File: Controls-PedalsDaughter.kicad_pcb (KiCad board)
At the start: 2 copper layers, 40 x 50 mm, 37 parts, among them J2 Accel Pos. Sensor, J3 PeripheralCANConnector, J4 Conn_01x02, J5 PeripheralCANConnector, U1 RI3-1205S, U2 PeripheralSOM, U3 TLV9301xDCK, U4 AMC1300BDWV, U5 TLV70130DBVR

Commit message: again
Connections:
- D1 pad 1: +3.3V -> +3V3
- D3 pad 1: +3.3V -> +3V3
- U2 pad 2: +3.3V -> +3V3
- U2 pad 9: +3.3V -> +3V3
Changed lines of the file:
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@@
 	(net 7 "+3V3PWR")
 	(net 8 "+3V3")
-	(net 9 "+3.3V")
-	(net 10 "Net-(D6-A)")
-	(net 11 "unconnected-(J2-Pin_2-Pad2)")
-	(net 12 "Net-(J2-Pin_5)")
-	(net 13 "/CAN_L")
-	(net 14 "/CAN_H")
-	(net 15 "/INP")
-	(net 16 "Net-(U3-+)")
-	(net 17 "unconnected-(U2-SPI1_NSS-Pad19)")
-	(net 18 "unconnected-(U2-I2C2_SCL-Pad8)")
-	(net 19 "unconnected-(U2-SPI1_MISO-Pad15)")
-	(net 20 "unconnected-(U2-VDDA(3.3V)-Pad10)")
-	(net 21 "unconnected-(U2-SPI2_NSS-Pad7)")
-	(net 22 "unconnected-(U2-GNDA-Pad12)")
-	(net 23 "unconnected-(U2-SPI1_SCK-Pad13)")
-	(net 24 "unconnected-(U2-SPI2_MOSI-Pad1)")
-	(net 25 "unconnected-(U2-SPI2_MISO-Pad3)")
-	(net 26 "unconnected-(U2-I2C1_SDA-Pad16)")
-	(net 27 "unconnected-(U2-I2C2_SDA-Pad6)")
-	(net 28 "unconnected-(U2-SPI2_SCK-Pad5)")
-	(net 29 "unconnected-(U2-SPI1_MOSI-Pad17)")
-	(net 30 "unconnected-(U2-I2C1_SCL-Pad14)")
-	(net 31 "unconnected-(U5-NC-Pad3)")
-	(net 32 "unconnected-(U5-NC-Pad2)")
+	(net 9 "Net-(D6-A)")
+	(net 10 "unconnected-(J2-Pin_2-Pad2)")
+	(net 11 "Net-(J2-Pin_5)")
+	(net 12 "/CAN_L")
+	(net 13 "/CAN_H")
+	(net 14 "/INP")
+	(net 15 "Net-(U3-+)")
+	(net 16 "unconnected-(U2-SPI1_NSS-Pad19)")
+	(net 17 "unconnected-(U2-I2C2_SCL-Pad8)")
+	(net 18 "unconnected-(U2-SPI1_MISO-Pad15)")
+	(net 19 "unconnected-(U2-VDDA(3.3V)-Pad10)")
+	(net 20 "unconnected-(U2-SPI2_NSS-Pad7)")
+	(net 21 "unconnected-(U2-GNDA-Pad12)")
+	(net 22 "unconnected-(U2-SPI1_SCK-Pad13)")
+	(net 23 "unconnected-(U2-SPI2_MOSI-Pad1)")
+	(net 24 "unconnected-(U2-SPI2_MISO-Pad3)")
+	(net 25 "unconnected-(U2-I2C1_SDA-Pad16)")
+	(net 26 "unconnected-(U2-I2C2_SDA-Pad6)")
+	(net 27 "unconnected-(U2-SPI2_SCK-Pad5)")
+	(net 28 "unconnected-(U2-SPI1_MOSI-Pad17)")
+	(net 29 "unconnected-(U2-I2C1_SCL-Pad14)")
+	(net 30 "unconnected-(U5-NC-Pad3)")
+	(net 31 "unconnected-(U5-NC-Pad2)")
 	(footprint "TestPoint:TestPoint_Pad_1.5x1.5mm"
 		(layer "F.Cu")
@@
 			(layers "*.Cu" "*.Mask")
 			(remove_unused_layers no)
-			(net 14 "/CAN_H")
+			(net 13 "/CAN_H")
 			(pinfunction "CAN_H")
 			(pintype "bidirectional")
@@
 			(layers "*.Cu" "*.Mask")
 			(remove_unused_layers no)
-			(net 13 "/CAN_L")
+			(net 12 "/CAN_L")
 			(pinfunction "CAN_L")
 			(pintype "bidirectional")
@@
 			(layers "F.Cu" "F.Paste" "F.Mask")
 			(roundrect_rratio 0.25)
-			(net 16 "Net-(U3-+)")
+			(net 15 "Net-(U3-+)")
 			(pinfunction "+")
 			(pintype "input")
@@
 			(layers "F.Cu" "F.Paste" "F.Mask")
 			(roundrect_rratio 0.25)
-			(net 32 "unconnected-(U5-NC-Pad2)")
+			(net 31 "unconnected-(U5-NC-Pad2)")
 			(pinfunction "NC")
 			(pintype "unspecified+no_connect")
@@
 			(layers "F.Cu" "F.Paste" "F.Mask")
 			(roundrect_rratio 0.25)
-			(net 31 "unconnected-(U5-NC-Pad3)")
+			(net 30 "unconnected-(U5-NC-Pad3)")
 			(pinfunction "NC")
 			(pintype "unspecified+no_connect")
@@
 			(layers "*.Cu" "*.Mask")
 			(remove_unused_layers no)
-			(net 11 "unconnected-(J2-Pin_2-Pad2)")
+			(net 10 "unconnected-(J2-Pin_2-Pad2)")
 			(pinfunction "Pin_2")
 			(pintype "passive+no_connect")
@@
 			(layers "*.Cu" "*.Mask")
 			(remove_unused_layers no)
-			(net 12 "Net-(J2-Pin_5)")
+			(net 11 "Net-(J2-Pin_5)")
 			(pinfunction "Pin_5")
 			(pintype "passive")
@@
 			(layers "*.Cu" "*.Mask")
 			(remove_unused_layers no)
-			(net 14 "/CAN_H")
+			(net 13 "/CAN_H")
 			(pinfunction "CAN_H")
 			(pintype "bidirectional")
@@
 			(layers "*.Cu" "*.Mask")
 			(remove_unused_layers no)
-			(net 13 "/CAN_L")
+			(net 12 "/CAN_L")
 			(pinfunction "CAN_L")
 			(pintype "bidirectional")
@@
 			(layers "F.Cu" "F.Paste" "F.Mask")
 			(roundrect_rratio 0.25)
-			(net 15 "/INP")
+			(net 14 "/INP")
 			(pinfunction "+")
 			(pintype "input")
@@
 			(layers "F.Cu" "F.Paste" "F.Mask")
 			(roundrect_rratio 0.25)
-			(net 10 "Net-(D6-A)")
+			(net 9 "Net-(D6-A)")
 			(pinfunction "A")
 			(pintype "passive")
@@
 			(layers "*.Cu" "*.Mask")
 			(remove_unused_layers no)
-			(net 15 "/INP")
+			(net 14 "/INP")
 			(pinfunction "Pin_2")
 			(pintype "passive")
@@
 			(layers "B.Cu" "B.Paste" "B.Mask")
 			(roundrect_rratio 0.25)
-			(net 9 "+3.3V")
+			(net 8 "+3V3")
 			(pinfunction "K")
 			(pintype "passive")
@@
 			(layers "B.Cu" "B.Paste" "B.Mask")
 			(roundrect_rratio 0.243902)
-			(net 16 "Net-(U3-+)")
+			(net 15 "Net-(U3-+)")
 			(pintype "passive")
 		)
@@
 			(layers "B.Cu" "B.Paste" "B.Mask")
 			(roundrect_rratio 0.243902)
-			(net 12 "Net-(J2-Pin_5)")
+			(net 11 "Net-(J2-Pin_5)")
 			(pintype "passive")
 		)
@@
 			(layers "B.Cu" "B.Paste" "B.Mask")
 			(roundrect_rratio 0.243902)
-			(net 16 "Net-(U3-+)")
+			(net 15 "Net-(U3-+)")
 			(pintype "passive")
 		)
@@
 			(layers "B.Cu" "B.Paste" "B.Mask")
 			(roundrect_rratio 0.243902)
-			(net 10 "Net-(D6-A)")
+			(net 9 "Net-(D6-A)")
 			(pintype "passive")
 		)
@@
 			(layers "B.Cu" "B.Paste" "B.Mask")
 			(roundrect_rratio 0.243902)
-			(net 15 "/INP")
+			(net 14 "/INP")
 			(pintype "passive")
 		)
@@
 		(fp_arc
 			(start 21.237742 18.612258)
-			(mid 20.300482 20.874999)
+			(mid 20.300481 20.874995)
 			(end 18.037742 21.812258)
 			(stroke
@@
 			(size 0.55 1.8)
 			(layers "B.Cu" "B.Paste" "B.Mask")
-			(net 24 "unconnected-(U2-SPI2_MOSI-Pad1)")
+			(net 23 "unconnected-(U2-SPI2_MOSI-Pad1)")
 			(pinfunction "SPI2_MOSI")
 			(pintype "passive+no_connect")
 		)
 		(pad "2" smd rect
-			(at 20.475 1.175 90)
+			(at 20.475 1.175 270)
 			(size 0.55 1.8)
 			(layers "B.Cu" "B.Paste" "B.Mask")
-			(net 9 "+3.3V")
+			(net 8 "+3V3")
 			(pinfunction "+3.3V")
 			(pintype "passive")
@@
 			(size 0.55 1.8)
 			(layers "B.Cu" "B.Paste" "B.Mask")
-			(net 25 "unconnected-(U2-SPI2_MISO-Pad3)")
+			(net 24 "unconnected-(U2-SPI2_MISO-Pad3)")
 			(pinfunction "SPI2_MISO")
 			(pintype "passive+no_connect")
@@
 			(size 0.55 1.8)
 			(layers "B.Cu" "B.Paste" "B.Mask")
-			(net 28 "unconnected-(U2-SPI2_SCK-Pad5)")
+			(net 27 "unconnected-(U2-SPI2_SCK-Pad5)")
 			(pinfunction "SPI2_SCK")
 			(pintype "passive+no_connect")
@@
 			(size 0.55 1.8)
 			(layers "B.Cu" "B.Paste" "B.Mask")
-			(net 27 "unconnected-(U2-I2C2_SDA-Pad6)")
+			(net 26 "unconnected-(U2-I2C2_SDA-Pad6)")
 			(pinfunction "I2C2_SDA")
 			(pintype "passive+no_connect")
@@
 			(size 0.55 1.8)
 			(layers "B.Cu" "B.Paste" "B.Mask")
-			(net 21 "unconnected-(U2-SPI2_NSS-Pad7)")
+			(net 20 "unconnected-(U2-SPI2_NSS-Pad7)")
 			(pinfunction "SPI2_NSS")
 			(pintype "passive+no_connect")
@@
 			(size 0.55 1.8)
 			(layers "B.Cu" "B.Paste" "B.Mask")
-			(net 18 "unconnected-(U2-I2C2_SCL-Pad8)")
+			(net 17 "unconnected-(U2-I2C2_SCL-Pad8)")
 			(pinfunction "I2C2_SCL")
 			(pintype "passive+no_connect")
 		)
 		(pad "9" smd rect
-			(at 16.175 -2.025 90)
+			(at 16.175 -2.025 270)
 			(size 0.55 1.8)
 			(layers "B.Cu" "B.Paste" "B.Mask")
-			(net 9 "+3.3V")
+			(net 8 "+3V3")
 			(pinfunction "+3.3V")
 			(pintype "output")
@@
 			(size 0.55 1.8)
 			(layers "B.Cu" "B.Paste" "B.Mask")
-			(net 20 "unconnected-(U2-VDDA(3.3V)-Pad10)")
+			(net 19 "unconnected-(U2-VDDA(3.3V)-Pad10)")
 			(pinfunction "VDDA(3.3V)")
 			(pintype "passive+no_connect")
@@
 			(size 0.55 1.8)
 			(layers "B.Cu" "B.Paste" "B.Mask")
-			(net 22 "unconnected-(U2-GNDA-Pad12)")
+			(net 21 "unconnected-(U2-GNDA-Pad12)")
 			(pinfunction "GNDA")
 			(pintype "output+no_connect")
@@
 			(size 0.55 1.8)
 			(layers "B.Cu" "B.Paste" "B.Mask")
-			(net 23 "unconnected-(U2-SPI1_SCK-Pad13)")
+			(net 22 "unconnected-(U2-SPI1_SCK-Pad13)")
 			(pinfunction "SPI1_SCK")
 			(pintype "passive+no_connect")
@@
 			(size 0.55 1.8)
 			(layers "B.Cu" "B.Paste" "B.Mask")
-			(net 30 "unconnected-(U2-I2C1_SCL-Pad14)")
+			(net 29 "unconnected-(U2-I2C1_SCL-Pad14)")
 			(pinfunction "I2C1_SCL")
 			(pintype "passive+no_connect")
@@
 			(size 0.55 1.8)
 			(layers "B.Cu" "B.Paste" "B.Mask")
-			(net 19 "unconnected-(U2-SPI1_MISO-Pad15)")
+			(net 18 "unconnected-(U2-SPI1_MISO-Pad15)")
 			(pinfunction "SPI1_MISO")
 			(pintype "passive+no_connect")
@@
 			(size 0.55 1.8)
 			(layers "B.Cu" "B.Paste" "B.Mask")
-			(net 26 "unconnected-(U2-I2C1_SDA-Pad16)")
+			(net 25 "unconnected-(U2-I2C1_SDA-Pad16)")
 			(pinfunction "I2C1_SDA")
 			(pintype "passive+no_connect")
@@
 			(size 0.55 1.8)
 			(layers "B.Cu" "B.Paste" "B.Mask")
-			(net 29 "unconnected-(U2-SPI1_MOSI-Pad17)")
+			(net 28 "unconnected-(U2-SPI1_MOSI-Pad17)")
 			(pinfunction "SPI1_MOSI")
 			(pintype "passive+no_connect")
@@
 			(size 0.55 1.8)
 			(layers "B.Cu" "B.Paste" "B.Mask")
-			(net 17 "unconnected-(U2-SPI1_NSS-Pad19)")
+			(net 16 "unconnected-(U2-SPI1_NSS-Pad19)")
 			(pinfunction "SPI1_NSS")
 			(pintype "passive+no_connect")
@@
 			(size 0.55 1.8)
 			(layers "B.Cu" "B.Paste" "B.Mask")
-			(net 13 "/CAN_L")
+			(net 12 "/CAN_L")
 			(pinfunction "CAN_L")
 			(pintype "passive")
@@
 			(size 0.55 1.8)
 			(layers "B.Cu" "B.Paste" "B.Mask")
-			(net 14 "/CAN_H")
+			(net 13 "/CAN_H")
 			(pinfunction "CAN_H")
 			(pintype "passive")
@@
 			(layers "B.Cu" "B.Paste" "B.Mask")
 			(roundrect_rratio 0.25)
-			(net 9 "+3.3V")
+			(net 8 "+3V3")
 			(pinfunction "K")
 			(pintype "passive")

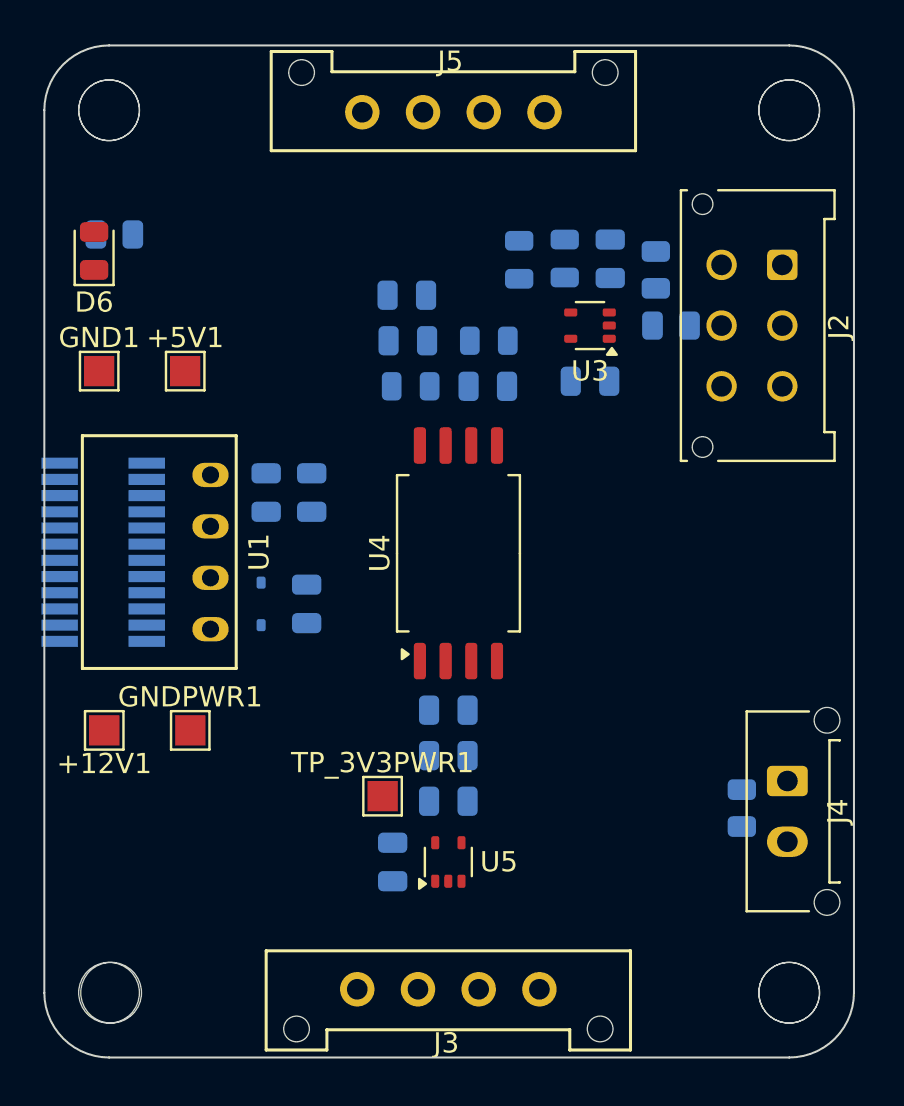
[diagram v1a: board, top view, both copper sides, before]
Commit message: Yuh
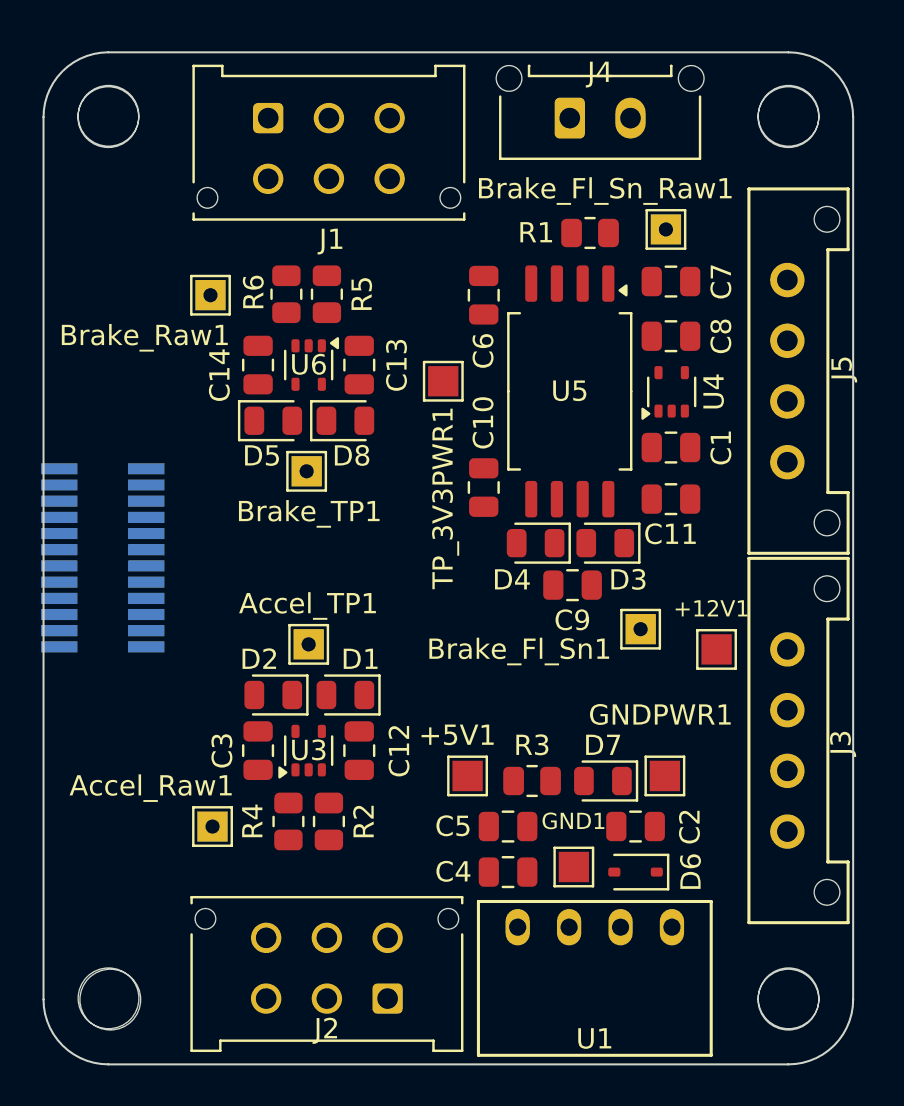
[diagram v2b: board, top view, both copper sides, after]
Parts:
- added Accel_Raw1: Accel_Raw_TP, TestPoint:TestPoint_THTPad_1.5x1.5mm_Drill0.7mm, F.Cu at (101.8, 76.5)
- added Accel_TP1: Accel, TestPoint:TestPoint_THTPad_1.5x1.5mm_Drill0.7mm, F.Cu at (106.6, 67.5)
- added Brake_Fl_Sn1: Brake_Fl_Sn_TP, TestPoint:TestPoint_THTPad_1.5x1.5mm_Drill0.7mm, F.Cu at (123.0, 66.8)
- added Brake_Fl_Sn_Raw1: Brake_Fl_Sn_Raw_TP, TestPoint:TestPoint_THTPad_1.5x1.5mm_Drill0.7mm, F.Cu at (124.2, 47.0)
- added Brake_Raw1: Brake_Raw_TP, TestPoint:TestPoint_THTPad_1.5x1.5mm_Drill0.7mm, F.Cu at (101.8, 50.2)
- added Brake_TP1: Brake, TestPoint:TestPoint_THTPad_1.5x1.5mm_Drill0.7mm, F.Cu at (106.5, 59.0)
- added C13: 0.1uf, Capacitor_SMD:C_0805_2012Metric, F.Cu at (109.1, 53.7)
- added C14: 1nf, Capacitor_SMD:C_0805_2012Metric, F.Cu at (104.1, 53.7)
- added D5: MBR, Diode_SMD:D_0805_2012Metric, F.Cu at (104.8, 56.5)
- added D8: MBR, Diode_SMD:D_0805_2012Metric, F.Cu at (108.4, 56.5)
- added J1: Brake Pos. Sensor, Connector_Molex:Molex_Micro-Fit_3.0_43045-0612_2x03_P3.00mm_Vertical, F.Cu at (104.6, 41.5)
- added R5: 8.2k, Resistor_SMD:R_0805_2012Metric, F.Cu at (107.5, 50.2)
- added R6: 22k, Resistor_SMD:R_0805_2012Metric, F.Cu at (105.5, 50.2)
- added U6: TLV9301xDCK, Package_TO_SOT_SMD:SOT-353_SC-70-5, F.Cu at (106.6, 53.7)
- C1: value 1nF -> 100nF; moved to F.Cu
- C10: value 1nF -> 1uF; moved to F.Cu
- C11: value 100nF -> 100uF; moved to F.Cu
- C12: value 0.1uf -> 1nf; moved to F.Cu
- C2, C4, C5, C6, C7, D1, D2, D3, D4, R1, R2, R3, R4: moved to F.Cu
- C3: value 1nf -> 0.1uf; moved to F.Cu
- C8: value 1uF -> 1nF; moved to F.Cu
- C9: value 100uF -> 1nF; moved to F.Cu
- D6: value SMD_0805 -> PESD15VL1BA; footprint Diode_SMD:D_0805_2012Metric -> Diode_SMD:D_SOD-323
- D7: value PESD15VL1BA -> SMD_0805; footprint Diode_SMD:D_SOD-323 -> Diode_SMD:D_0805_2012Metric; moved to F.Cu
- U4: value AMC1300BDWV -> TLV70130DBVR; footprint Package_SO:SOIC-8_7.5x5.85mm_P1.27mm -> Package_TO_SOT_SMD:SOT-353_SC-70-5
- U5: value TLV70130DBVR -> AMC1300BDWV; footprint Package_TO_SOT_SMD:SOT-353_SC-70-5 -> Package_SO:SOIC-8_7.5x5.85mm_P1.27mm
- moved J2 41.2 mm to (110.5, 85.0), turned to 180 degrees
- moved D6 40.7 mm to (122.8, 78.8), turned to 180 degrees
- moved J4 34.5 mm to (119.5, 41.5), turned to 0 degrees
- moved R3 34.0 mm to (117.6, 74.2), turned to 0 degrees
- moved GND1 33.9 mm to (119.7, 78.5), turned to 90 degrees
- moved R4 32.7 mm to (105.6, 76.2), turned to -90 degrees
- moved +12V1 30.5 mm to (126.8, 67.8), turned to 0 degrees
- moved C3 29.9 mm to (104.1, 72.8), turned to 90 degrees
- moved R2 29.8 mm to (107.6, 76.2), turned to -90 degrees
- moved R1 29.4 mm to (120.5, 47.2), turned to 180 degrees
- moved U1 26.5 mm to (120.7, 81.5), turned to 180 degrees
- moved D2 25.9 mm to (104.8, 70.0), turned to 180 degrees
- moved C7 25.9 mm to (124.5, 49.6)
- moved U3 25.2 mm to (106.6, 72.8), turned to 90 degrees
- moved +5V1 24.4 mm to (114.5, 74.0), turned to 90 degrees
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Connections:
- C1 pad 1: /Brake -> +12V
- C1 pad 2: GND -> GNDPWR
- C10 pad 1: +3V3PWR -> +3V3
- C10 pad 2: GNDPWR -> GND
- C11 pad 1: +12V -> +3V3
- C11 pad 2: GNDPWR -> GND
- C12 pad 2: +5V -> /Accel
- C3 pad 2: /Accel -> +5V
- C8 pad 1: +3V3 -> +3V3PWR
- C8 pad 2: GND -> GNDPWR
- C9 pad 1: +3V3 -> /Brake_Fl
- D3 pad 2: /Brake -> /Brake_Fl
- D4 pad 1: /Brake -> /Brake_Fl
- D6 pad 1: GND -> GNDPWR
- D6 pad 2: Net-(D6-A) -> +12V
- D7 pad 1: GNDPWR -> GND
- D7 pad 2: +12V -> Net-(D7-A)
- J4 pad 2: /INP -> /Brake Fluid Sensor/INP
- R1 pad 1: /INP -> /Brake Fluid Sensor/INP
- R3 pad 2: Net-(D6-A) -> Net-(D7-A)
- U2 pad 19: unconnected-(U2-SPI1_NSS-Pad19) -> /Brake_Fl
- U2 pad 20: /Brake -> /Brake_Pot
- U4 pad 1: +3V3PWR -> +12V
- U4 pad 2: /INP -> unconnected-(U4-NC-Pad2)
- U4 pad 3: GNDPWR -> unconnected-(U4-NC-Pad3)
- U4 pad 5: GND -> +3V3PWR
- U5 pad 1: +12V -> +3V3PWR
- U5 pad 2: unconnected-(U5-NC-Pad2) -> /Brake Fluid Sensor/INP
- U5 pad 3: unconnected-(U5-NC-Pad3) -> GNDPWR
- U5 pad 5: +3V3PWR -> GND
